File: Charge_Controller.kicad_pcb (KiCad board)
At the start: 2 copper layers, 134.6 x 76.2 mm, 160 parts, among them J1 SOLAR, J10 Conn_01x01_Female, J11 Conn_01x01_Female, J12 Conn_01x01_Female, J13 Conn_01x01_Female, J14 Conn_01x01_Female, J15 Conn_01x01_Female, J16 Conn_01x01_Female, J17 Conn_01x01_Female, J18 Conn_01x01_Female, J19 Conn_01x01_Female, J2 Conn_01x01_Female, J20 Conn_01x01_Female, J21 Conn_01x01_Female, J22 Conn_01x01_Female, J23 Conn_01x01_Female, J24 Conn_01x01_Female, J25 Conn_01x01_Female, J26 Conn_01x01_Female, J27 Conn_01x01_Female, J28 Conn_01x01_Female, J29 Conn_01x01_Female, J3 Conn_01x01_Female, J30 Conn_01x01_Female, J31 Conn_01x01_Female, J32 Conn_01x01_Female, J33 Conn_01x01_Female, J34 Conn_01x01_Female, J36 FAN, J38 I2C_CON, J4 Conn_01x01_Female, J5 Conn_01x01_Female, J6 Conn_01x01_Female, J7 Conn_01x01_Female, J8 BATT, J9 USB_OTG, Q1 CSD19505, Q2 CSD19505, Q3 CSD19505, Q4 Si2306, Q5 2N3904, Q6 2N3904, Q7 PMOS-100V-78A, Q8 PMOS-100V-78A, Q9 Si2306, SW1 RIGHT, SW2 LEFT, SW3 BACK, SW4 SELECT, U1 Hall Amp Sense, U10 ADS1015, U11 NUP4202, U12 PCF8574, U2 B1212, U3 AMS1117-5.0, U4 AMS1117-3.3, U5 XL7005A, U6 XL7005A, U7 IR2104, U8 ESP32-WROOM-32, U9 CH340C

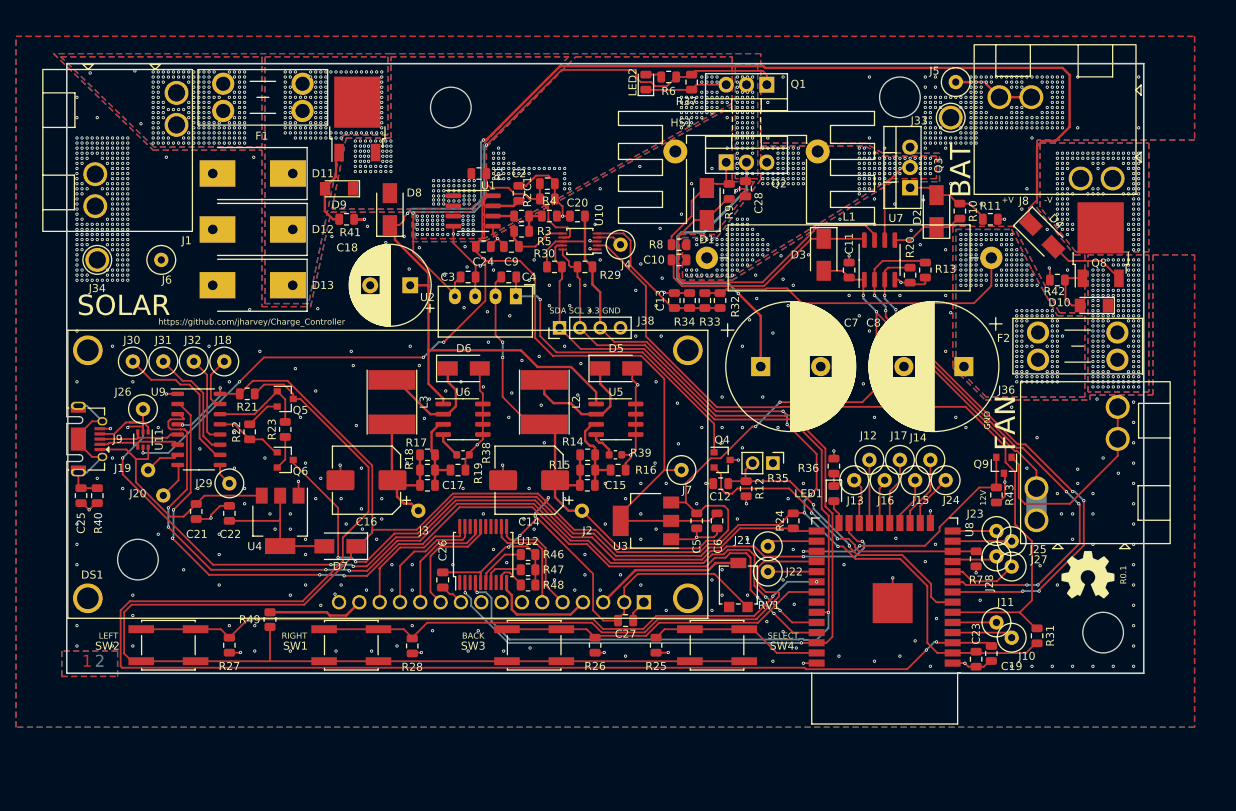
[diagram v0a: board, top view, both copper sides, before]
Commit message: Draft layout, still needs a bunch, but everything is connected.
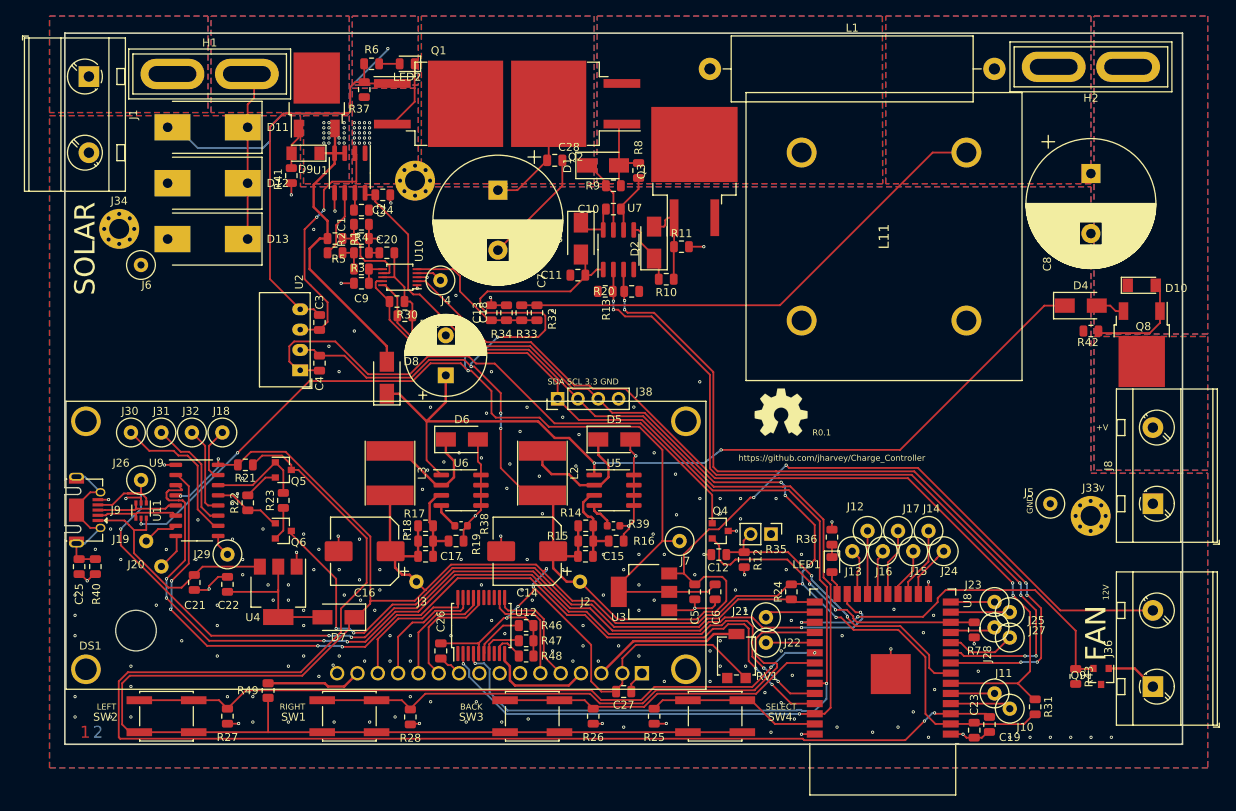
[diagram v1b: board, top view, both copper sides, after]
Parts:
- added H1: Holder, Fuse_Holder:Fuse_Blade_C2935871, F.Cu at (79.7, 69.1)
- added H2: Holder, Fuse_Holder:Fuse_Blade_C2935871, F.Cu at (199.1, 68.2)
- added L11: 7443783533650, 7443783533650_inductor:7443783533650, F.Cu at (158.3, 79.0)
- C28: value 100nf -> 470nf
- F1, F2: value 35A -> 25A; footprint Fuse:Fuseholder_Blade_Mini_Keystone_3568 -> Symbol:ESD-Logo_6.6x6mm_SilkScreen; moved to B.Cu
- HS1: value Heatsink -> 100x41x8mm Aluminum Heat Sink; footprint Heatsink:Heatsink_Stonecold_HS-132_32x14mm_2xFixation1.5mm -> MountingHole:MountingHole_2.5mm_Pad_Via; moved to B.Cu
- J1, J36, J8: footprint Phoenix_10.16_terminal_1709681:Phoenix_10.16_terminal_1709681 -> TerminalBlock_MetzConnect:TerminalBlock_MetzConnect_Type703_RT10N02HGLU_1x02_P9.52mm_Horizontal
- J33, J34: footprint TestPoint:TestPoint_Loop_D3.50mm_Drill0.9mm_Beaded -> MountingHole:MountingHole_2.5mm_Pad_Via
- Q1, Q2, Q3: footprint Package_TO_SOT_THT:TO-220-3_Vertical -> Package_TO_SOT_SMD:TO-263-2
- moved F2 117.5 mm to (84.6, 73.3)
- moved F1 108.5 mm to (194.5, 74.0), turned to 180 degrees
- moved J5 54.0 mm to (189.4, 122.9)
- moved J33 52.8 mm to (194.4, 124.4)
- moved LOGO1 43.4 mm to (155.7, 111.4)
- moved HS1 41.6 mm to (110.0, 82.5), turned to 180 degrees
- moved J8 41.0 mm to (202.2, 122.9), turned to 90 degrees
- moved R37 40.9 mm to (103.6, 71.1)
- moved R13 40.1 mm to (133.8, 96.3), turned to 0 degrees
- moved C7 39.6 mm to (120.3, 83.7), turned to -90 degrees
- moved R11 38.8 mm to (143.3, 90.7)
- moved Q1 38.6 mm to (112.9, 72.9), turned to 0 degrees
- moved R10 37.7 mm to (141.4, 94.8), turned to 0 degrees
- moved R6 37.2 mm to (104.5, 67.9), turned to 180 degrees
- moved D2 35.5 mm to (139.9, 90.2)
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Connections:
- net Net-(LED2-Pad2) renamed /L2
- C16 pad 1: /3.3V -> +3.3VA
- C17 pad 1: /3.3V -> +3.3VA
- HS1 pad 1: (no net) -> GND
- J3 pad 1: /3.3V -> +3.3VA
- J36 pad 1: /12V -> Net-(Q9-Pad1)
- J36 pad 2: Net-(J36-Pad2) -> /12V
- J8 pad 1: /B+ -> GND
- J8 pad 2: GND -> /B+
- L3 pad 2: /3.3V -> +3.3VA
- Q9 pad 1: Net-(J36-Pad2) -> Net-(Q9-Pad1)
- R17 pad 1: /3.3V -> +3.3VA
- R18 pad 1: /3.3V -> +3.3VA
- U1 pad 1: /S+Polarity -> /S+Fused2
- U1 pad 2: /S+Polarity -> /S+Fused2
- U1 pad 3: /S+Fused2 -> /S+Polarity
- U1 pad 4: /S+Fused2 -> /S+Polarity
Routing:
- net /S+B+1A: track 172.1 -> 112.1 mm
- net /12V: track 161.5 -> 214.5 mm
- net /S+Polarity: track 0.00 -> 39.6 mm, vias 99 -> 17
- net +3.3VA: track 398.5 -> 437.7 mm
- net Net-(D1-Pad1): track 42.4 -> 9.58 mm
- net Net-(C4-Pad2): track 40.1 -> 72.6 mm, vias 1 -> 0
- net /GPIO32: track 67.5 -> 98.3 mm
- net /GPIO33: track 70.4 -> 97.7 mm
- net Net-(J36-Pad2): track 26.7 -> 0.00 mm
- net Net-(C3-Pad1): track 75.0 -> 48.8 mm, vias 2 -> 0
- net /S+Fused3: track 40.9 -> 14.8 mm, vias 64 -> 0
- net Net-(C10-Pad1): track 29.1 -> 5.92 mm
- net /B+Fused: track 41.2 -> 63.5 mm, vias 200 -> 0
- net GND: track 131.5 -> 152.6 mm, vias 765 -> 198
- net /SDA: track 124.8 -> 145.8 mm
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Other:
- board size 134.6 x 76.2 mm -> 139.7 x 88.9 mm
- board text added: "heat sink"
- board text removed: "BAT"
